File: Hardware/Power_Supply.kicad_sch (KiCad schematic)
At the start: 66 parts, among them IC1 EA3036QBR, IC10 HY2213-BB3A, IC11 HY2213-BB3A, IC12 HY2213-BB3A, IC13 HY2213-BB3A, IC2 TPS5450DDAR, Q2 AO3401A, Q3 AO3400, Q4 AO3400, Q5 AO3400, Q6 AO3400

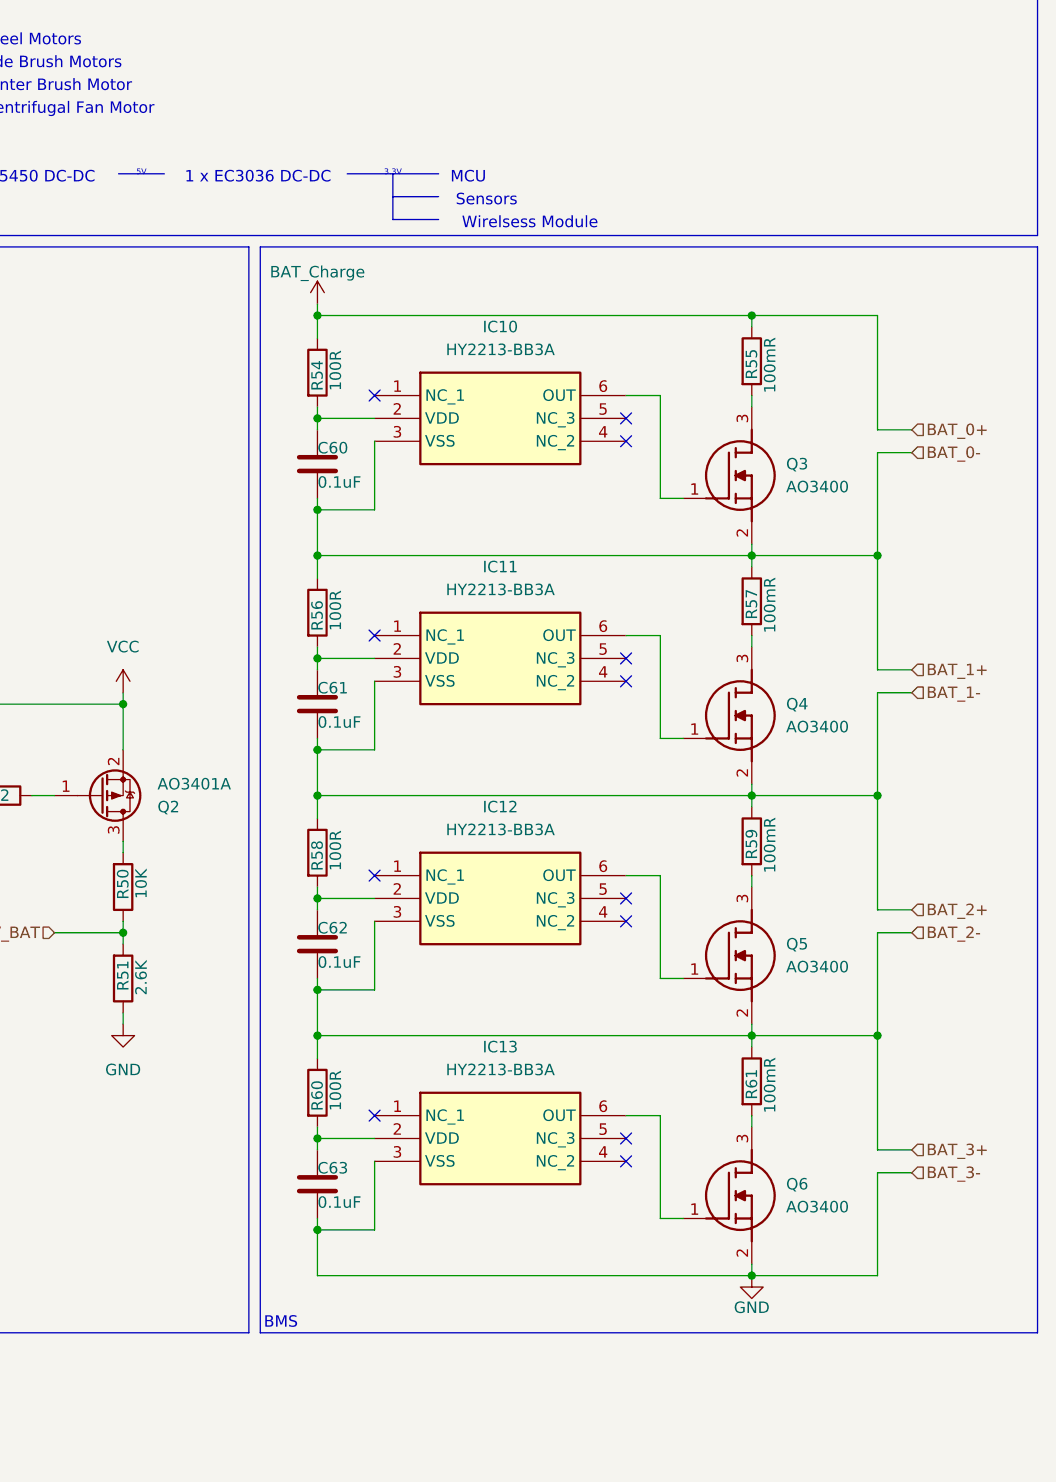
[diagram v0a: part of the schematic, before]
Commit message: Update SCH
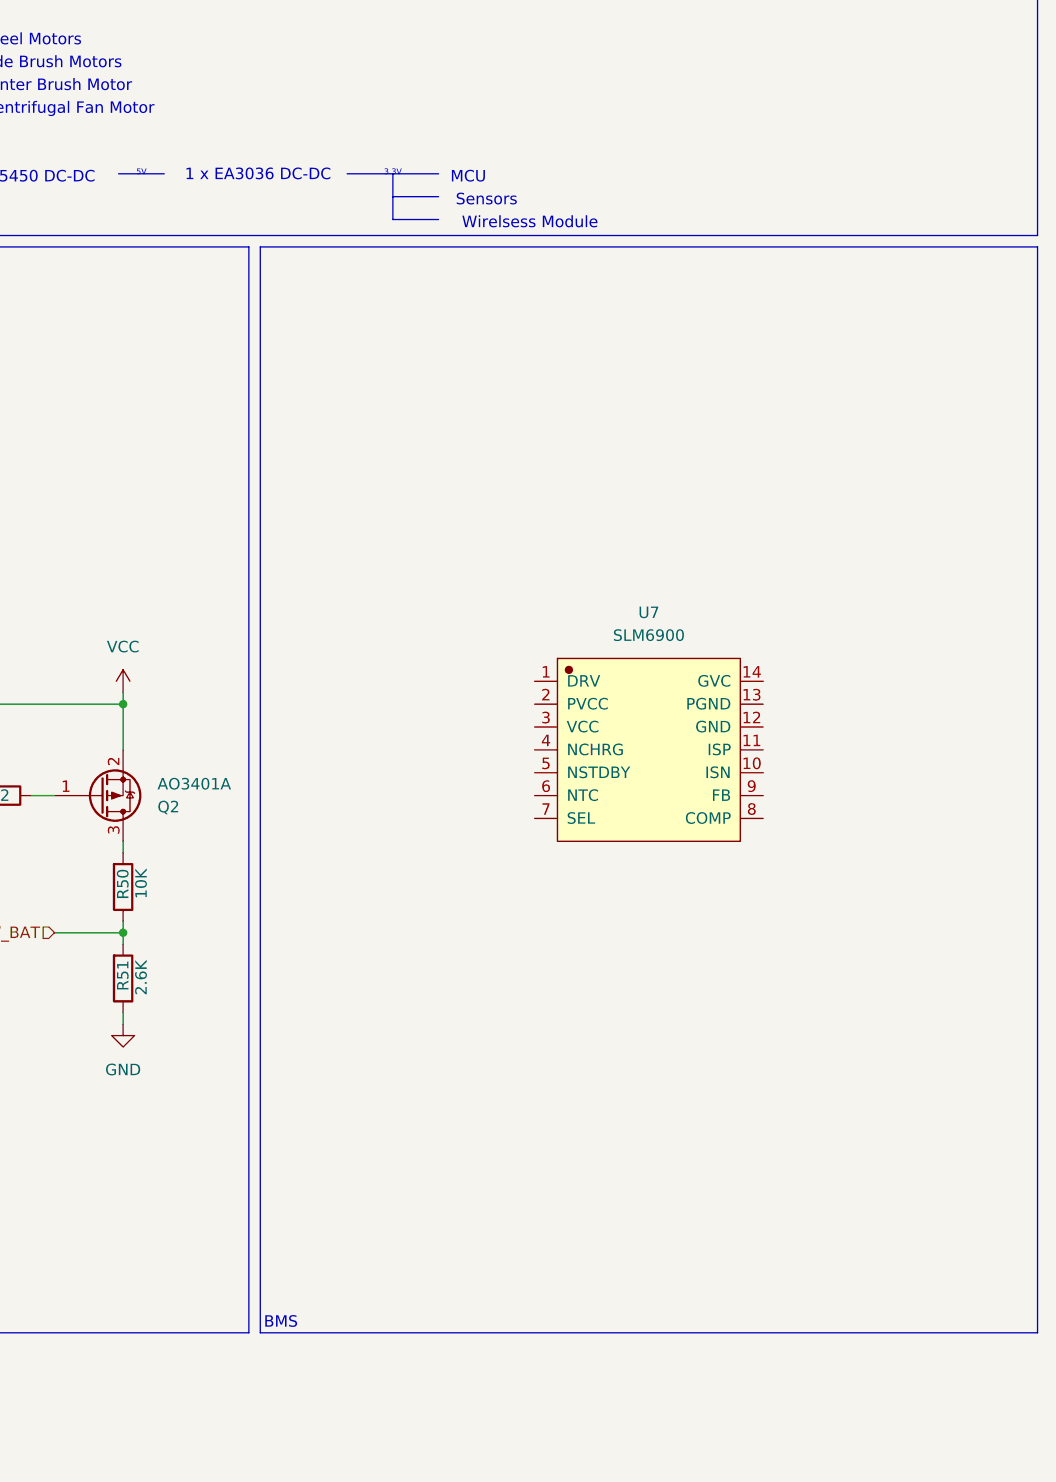
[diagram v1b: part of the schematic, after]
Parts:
- removed C60, C61, C62, C63: 0.1uF, symbol Device:C
- removed IC10, IC11, IC12, IC13: HY2213-BB3A, SOT95P280X140-6N, symbol SamacSys_Parts:HY2213-BB3A
- removed Q3, Q4, Q5, Q6: AO3400, SOT95P280X125-3N, symbol SamacSys_Parts:AO3400
- removed R54, R56, R58, R60: 100R, symbol Device:R
- removed R55, R57, R59, R61: 100mR, symbol Device:R
- added U7: SLM6900, SamacSys_Parts:TSSOP-14_L5.0-W4.4-P0.65-LS6.4-BL, symbol SamacSys_Parts:SLM6900
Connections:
- no-connect marks 15 -> 3
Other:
- note added: "1 x EA3036 DC-DC"
- note removed: "1 x EC3036 DC-DC"

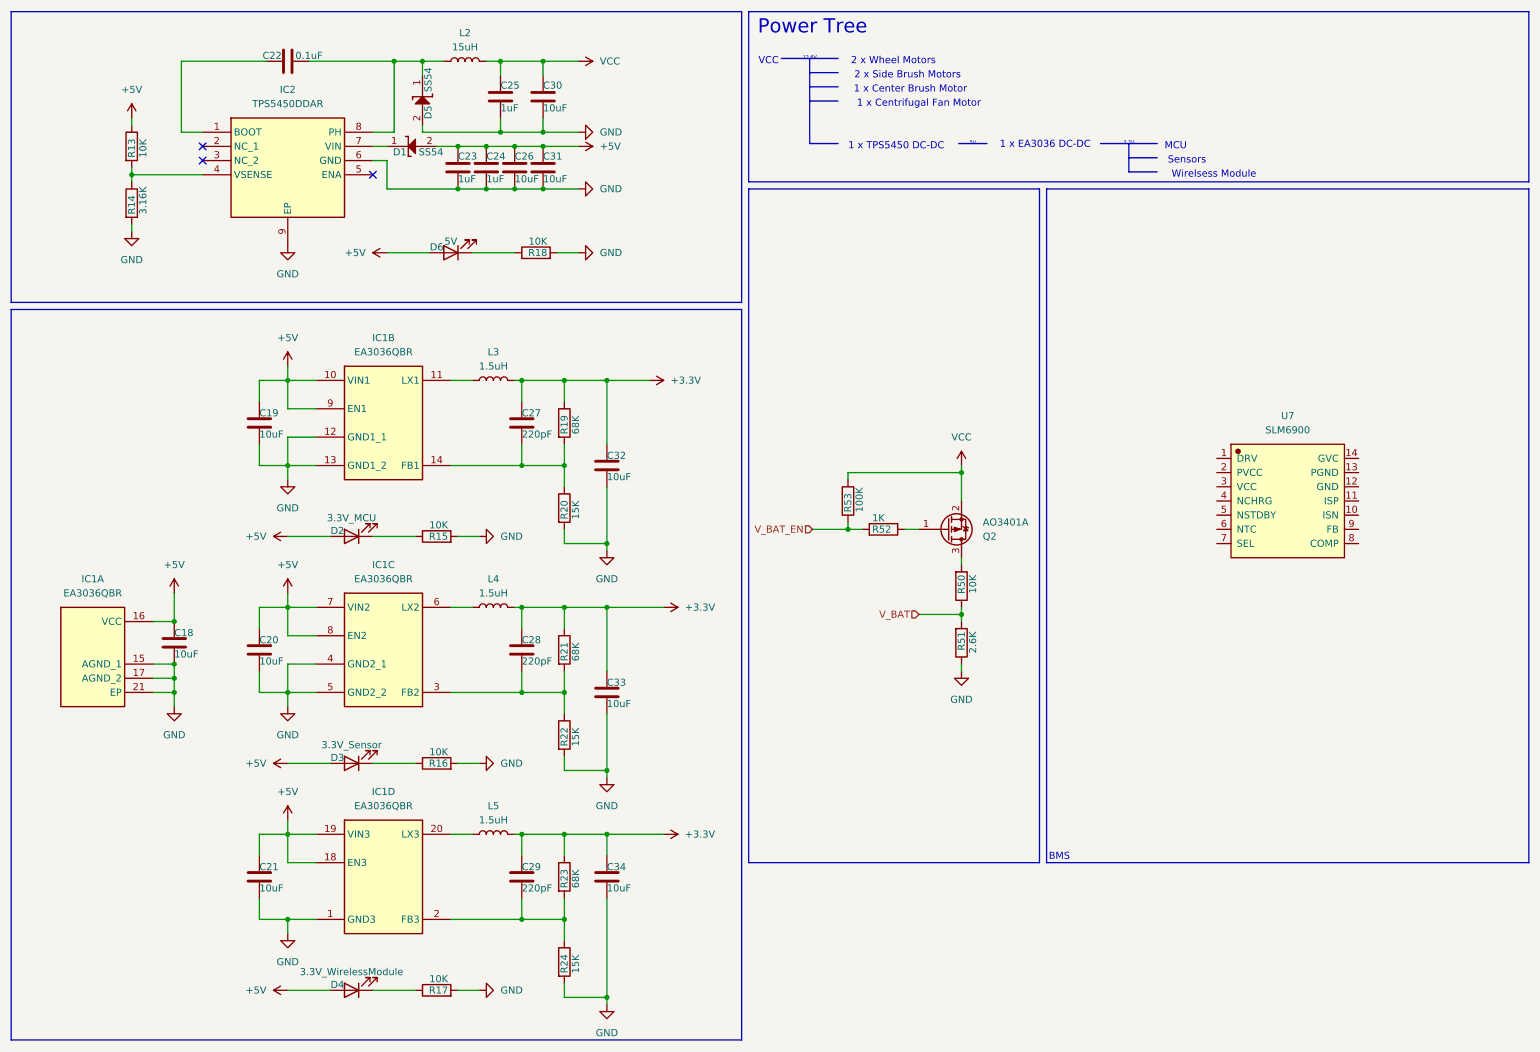
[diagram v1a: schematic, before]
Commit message: Update PCB
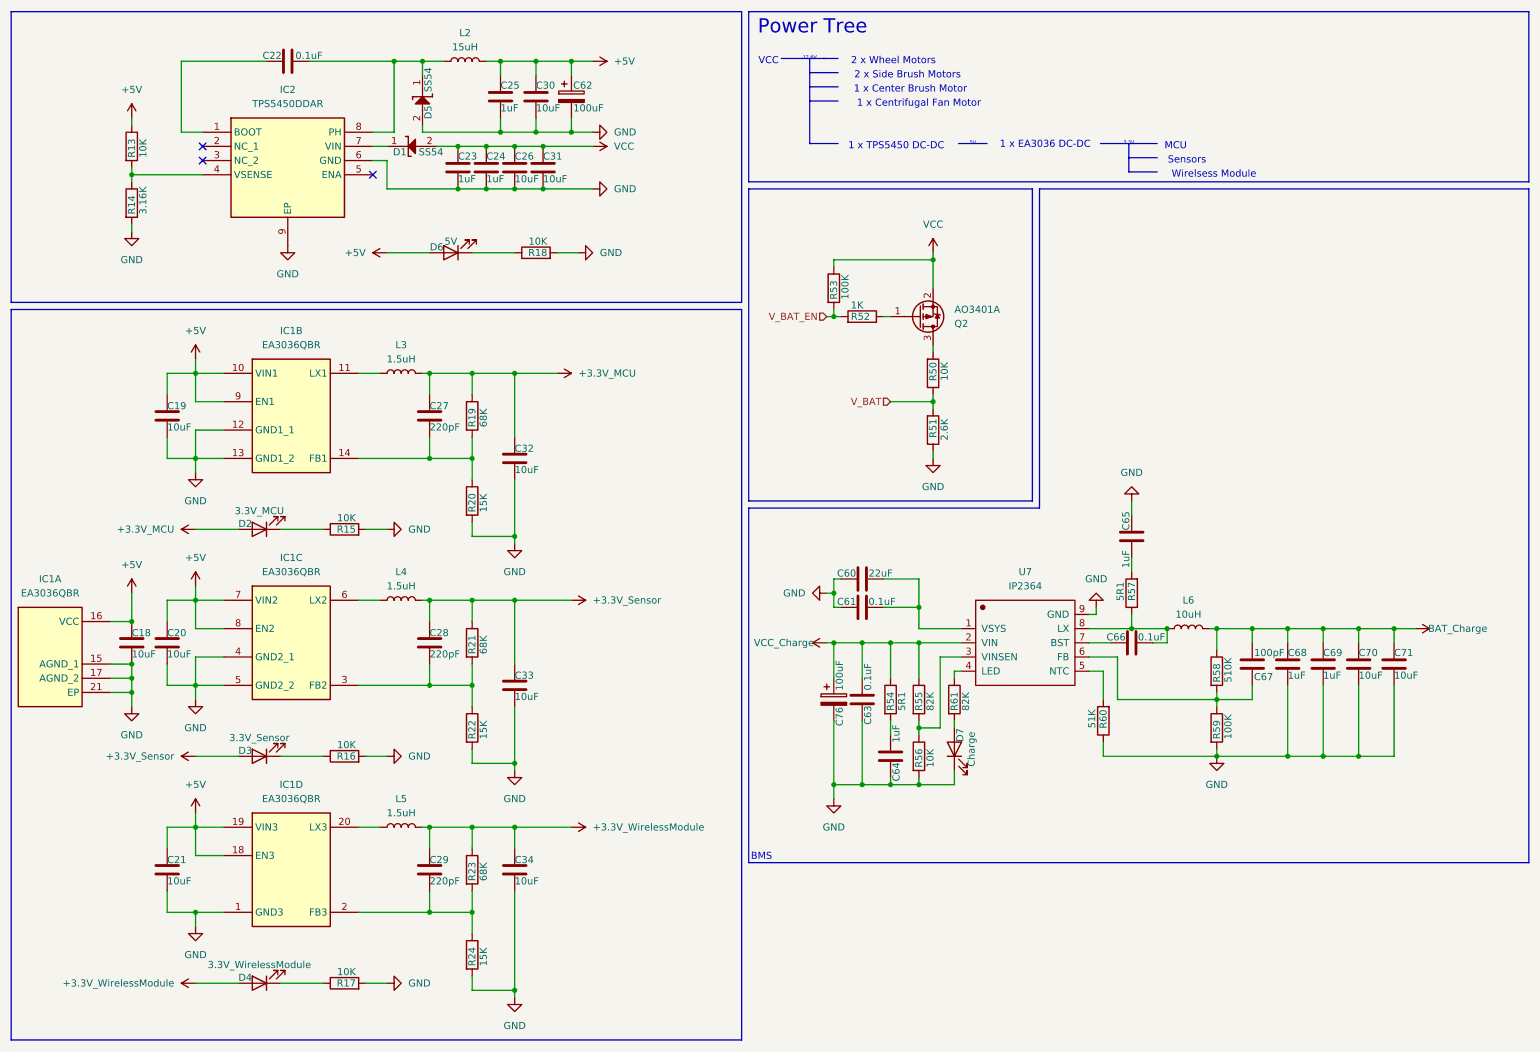
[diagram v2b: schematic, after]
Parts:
- removed U7: SLM6900, SamacSys_Parts:TSSOP-14_L5.0-W4.4-P0.65-LS6.4-BL, symbol SamacSys_Parts:SLM6900
- added C60: 22uF, Capacitor_SMD:C_0603_1608Metric, symbol Library:C
- added C61, C63, C66: 0.1uF, Capacitor_SMD:C_0603_1608Metric, symbol Library:C
- added C62, C76: 100uF, Capacitor_SMD:CP_Elec_6.3x7.7, symbol Library:C_Polarized
- added C64, C65, C68, C69: 1uF, Capacitor_SMD:C_0603_1608Metric, symbol Library:C
- added C67: 100pF, Capacitor_SMD:C_0603_1608Metric, symbol Library:C
- added C70, C71: 10uF, Capacitor_SMD:C_1206_3216Metric, symbol Library:C
- added D7: Charge, LED_SMD:LED_0603_1608Metric, symbol Library:LED
- added L6: 10uH, Inductor_SMD:L_Cenker_CKCS8060, symbol Library:L
- added R54, R57: 5R1, Resistor_SMD:R_0603_1608Metric, symbol Library:R
- added R55, R61: 82K, Resistor_SMD:R_0603_1608Metric, symbol Library:R
- added R56: 10K, Resistor_SMD:R_0603_1608Metric, symbol Library:R
- added R58: 510K, Resistor_SMD:R_0603_1608Metric, symbol Library:R
- added R59: 100K, Resistor_SMD:R_0603_1608Metric, symbol Library:R
- added R60: 51K, Resistor_SMD:R_0603_1608Metric, symbol Library:R
- added U7: IP2364, kicad_lceda:ESOP-8_L4.9-W3.9-P1.27-LS6.0-BL-EP-3, symbol Library:IP2364
- C18, C19, C20, C21, C22, C27, C28, C29, C32, C33, C34: footprint (none) -> Capacitor_SMD:C_0603_1608Metric; symbol Device:C -> Library:C
- C23, C24, C25, C26, C30, C31: footprint (none) -> Capacitor_SMD:C_1206_3216Metric; symbol Device:C -> Library:C
- D1, D5: symbol SamacSys_Parts:SS54 -> Library:SS54
- D2, D3, D4, D6: footprint (none) -> LED_SMD:LED_0603_1608Metric; symbol Device:LED -> Library:LED
- IC1: symbol SamacSys_Parts:EA3036QBR -> Library:EA3036QBR
- IC2: symbol SamacSys_Parts:TPS5450DDAR -> Library:TPS5450DDAR
- L2: footprint (none) -> Inductor_SMD:L_Cenker_CKCS8060; symbol Device:L -> Library:L
- L3, L4, L5: footprint (none) -> Inductor_SMD:L_1210_3225Metric; symbol Device:L -> Library:L
- Q2: symbol Transistor_FET:AO3401A -> Library:AO3401A
- R13, R14, R15, R16, R17, R18, R19, R20, R21, R22, R23, R24, R50, R51, R52, R53: footprint (none) -> Resistor_SMD:R_0603_1608Metric; symbol Device:R -> Library:R
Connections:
- net +5V: now also C25.1, C30.1, L2.2, C62.1; no longer C23.1, C24.1, C26.1, C31.1, D1.2 (A), D2.2 (A), D3.2 (A), D4.2 (A)
- net GND: now also C60.1, C61.1, C62.2, C63.1, C64.1, C65.1, C68.2, C69.2, C70.2, C71.2, C76.2, D7.1 (K), R56.2, R59.2, R60.1, U7.9 (GND)
- net VCC: now also C23.1, C24.1, C26.1, C31.1, D1.2 (A); no longer C25.1, C30.1, L2.2
- removed net +3.3V: C27.1, C28.1, C29.1, C32.1, C33.1, C34.1, L3.2, L4.2, L5.2, R19.1, R21.1, R23.1
- new net: C60.2, C61.2, U7.1 (VSYS)
- new net: C66.1, U7.7 (BST)
- new net: C66.2, L6.1, R57.1, U7.8 (LX)
- new net: C64.2, R54.2
- new net: C67.1, R58.2, R59.1, U7.6 (FB)
- new net: R55.2, R56.1, U7.3 (VINSEN)
- new net: D7.2 (A), R61.2
- new net: C65.2, R57.2
- new net: R60.2, U7.5 (NTC)
- new net: R61.1, U7.4 (LED)
- new net +3.3V_MCU: C27.1, C32.1, D2.2 (A), L3.2, R19.1
- new net +3.3V_Sensor: C28.1, C33.1, D3.2 (A), L4.2, R21.1
- new net +3.3V_WirelessModule: C29.1, C34.1, D4.2 (A), L5.2, R23.1
- new net BAT_Charge: C67.2, C68.1, C69.1, C70.1, C71.1, L6.2, R58.1
- new net VCC_Charge: C63.2, C76.1, R54.1, R55.1, U7.2 (VIN)
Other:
- moved on the sheet: C18, C19, C20, C21, C27, C28, C29, C30, C32, C33, C34, D2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
